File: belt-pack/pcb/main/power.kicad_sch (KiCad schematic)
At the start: 6 parts, among them U2 TP4056

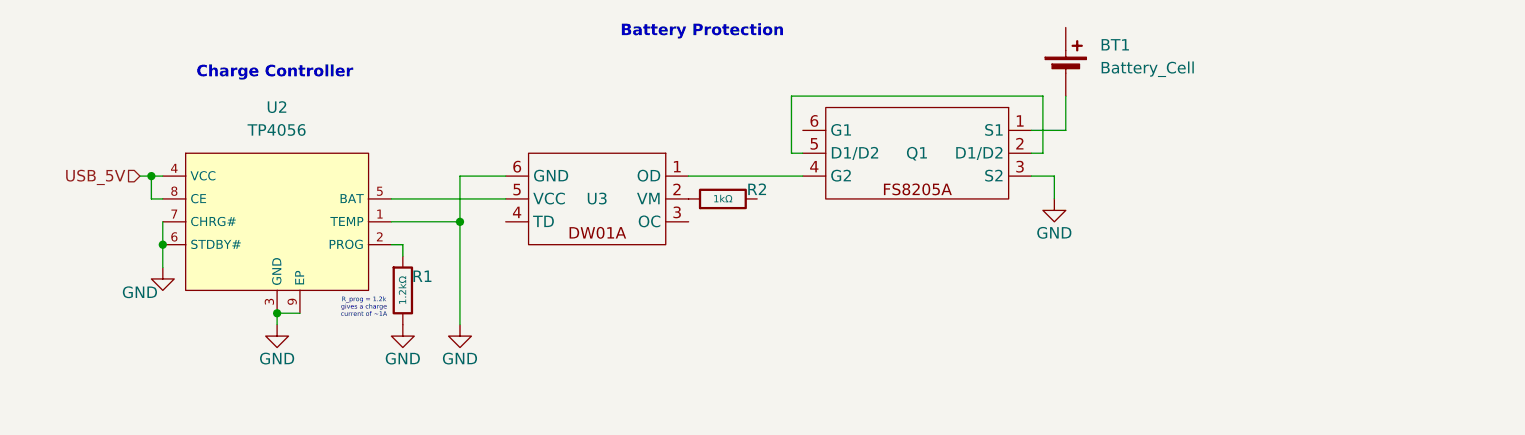
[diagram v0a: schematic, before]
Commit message: Nearly finished with battery circuitry
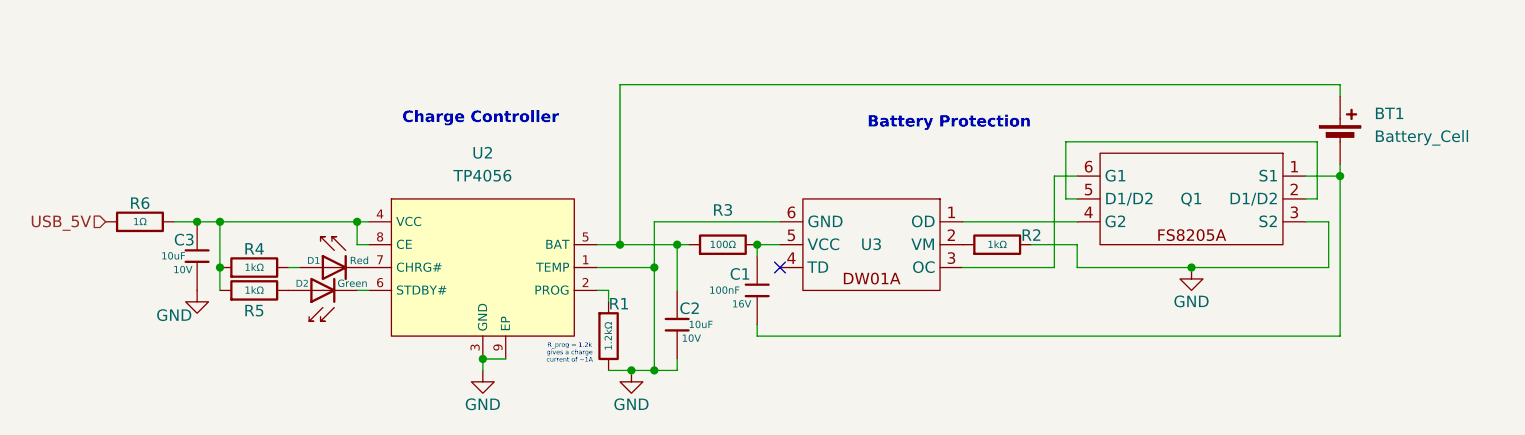
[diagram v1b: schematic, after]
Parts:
- added C1: 100nF, PCM_JLCPCB:C_0402, symbol PCM_JLCPCB-Capacitors:0402,100nF
- added C2, C3: 10uF, PCM_JLCPCB:C_0603, symbol PCM_JLCPCB-Capacitors:0603,10uF
- added D1: Red, PCM_JLCPCB:D_0603, symbol PCM_JLCPCB-Diodes:LED,0603,Red
- added D2: Green, PCM_JLCPCB:D_0805, symbol PCM_JLCPCB-Diodes:LED,0805,Green
- added R3: 100Ω, PCM_JLCPCB:R_0402, symbol PCM_JLCPCB-Resistors:0402,100Ω
- added R4, R5: 1kΩ, PCM_JLCPCB:R_0402, symbol PCM_JLCPCB-Resistors:0402,1kΩ
- added R6: 1Ω, PCM_JLCPCB:R_1206, symbol PCM_JLCPCB-Resistors:1206,1Ω
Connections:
- net GND: now also R2.2, C2.2, C3.2; no longer U2.6 (STDBY#), U2.7 (CHRG#)
- net USB_5V: now also R6.1; no longer U2.4 (VCC), U2.8 (CE)
- net at BT1.2 (-), Q1.1 (S1): now also C1.2
- net at Q1.6 (G1): now also U3.3 (OC)
- net at U2.5 (BAT): now also BT1.1 (+), C2.1, R3.1; no longer U3.5 (VCC)
- new net: C3.1, R4.1, R5.1, R6.2, U2.4 (VCC), U2.8 (CE)
- new net: D2.2, R5.2
- new net: C1.1, R3.2, U3.5 (VCC)
- new net: D1.2, R4.2
- new net: D2.1, U2.6 (STDBY#)
- new net: D1.1, U2.7 (CHRG#)
- no-connect marks 0 -> 1
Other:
- moved on the sheet: BT1, Q1, R1, R2, U2, U3
